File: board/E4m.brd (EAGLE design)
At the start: 49.4 x 100.1 mm, 76 parts, among them IC1 MCP23017SS, Q1 IRL540, Q2 IRL540, Q3 IRL540

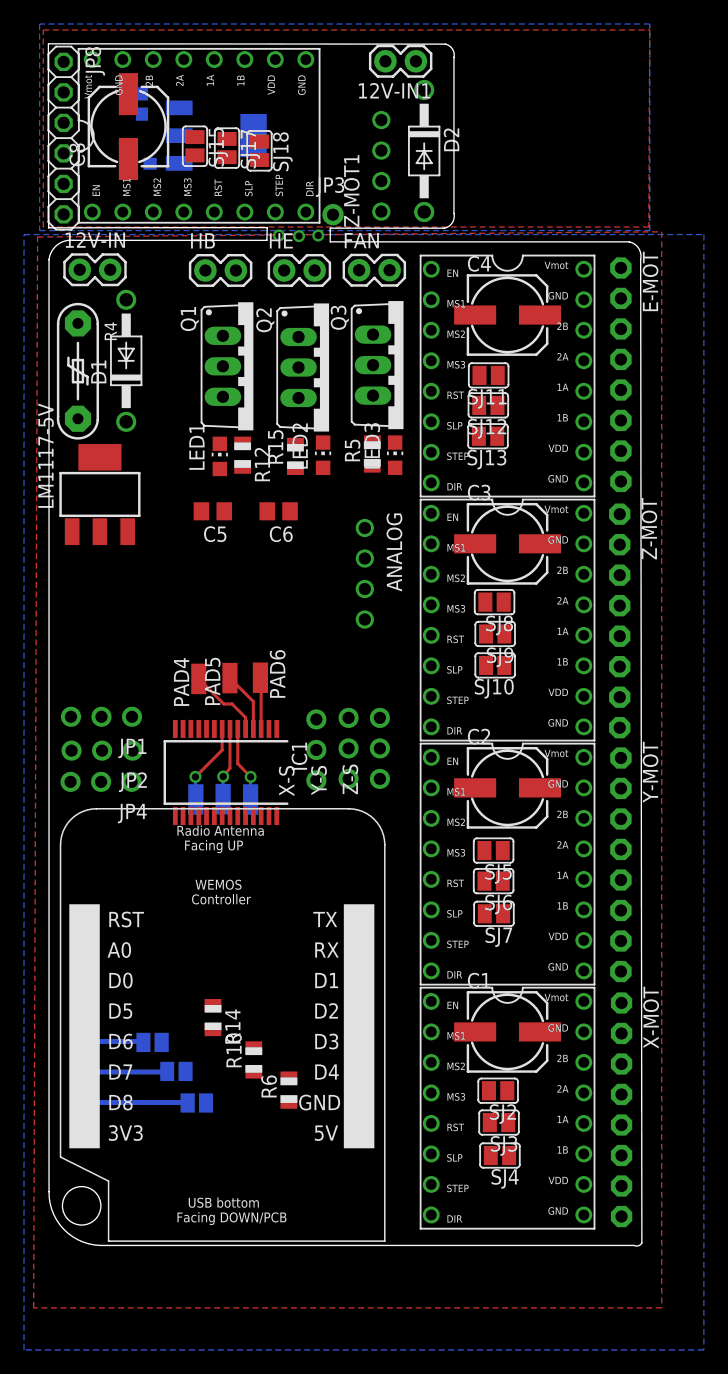
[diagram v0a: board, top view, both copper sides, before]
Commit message: 100% routed..... to clean before raster...
yup
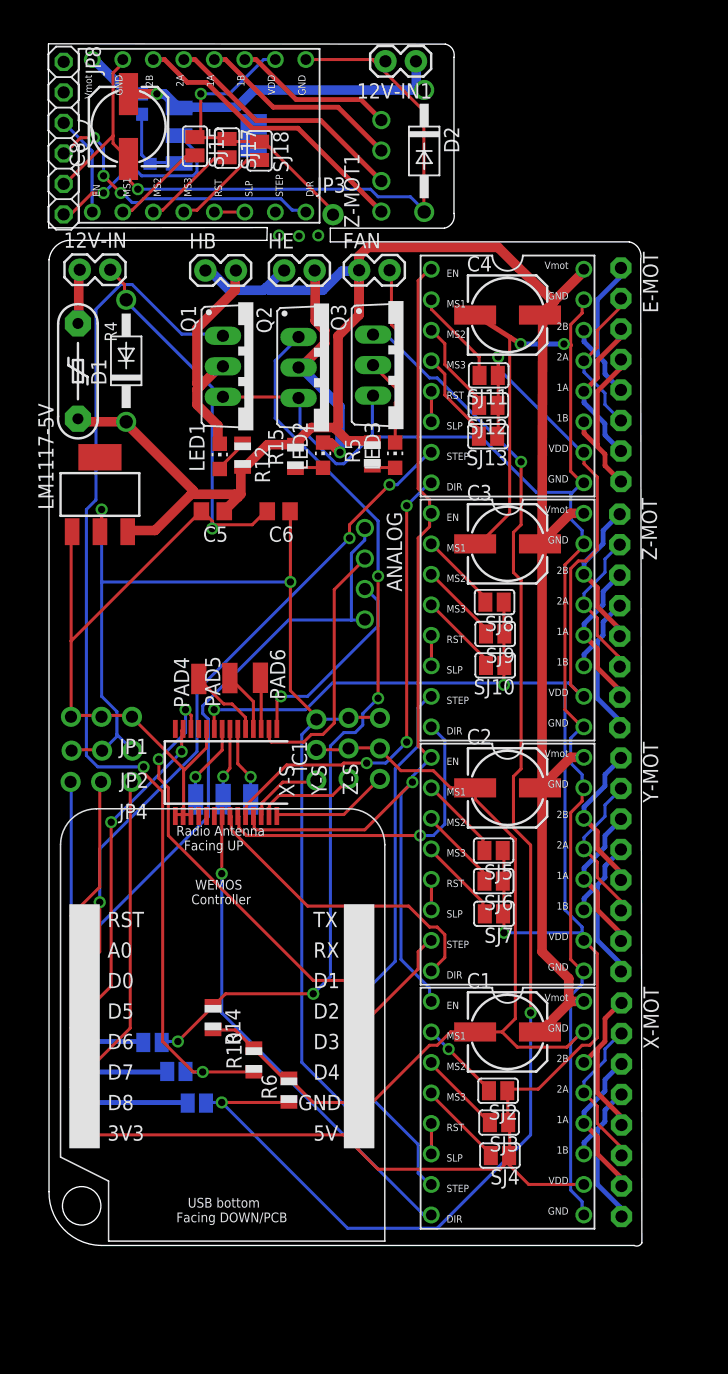
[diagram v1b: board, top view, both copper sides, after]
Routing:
- net GND: track 0.23 -> 310.8 mm, vias 0 -> 3
- net 3V3: track 0.18 -> 186.3 mm, vias 0 -> 4
- net 12V: track 0.00 -> 171.6 mm
- net N$27: track 0.00 -> 114.4 mm, vias 0 -> 3
- net 5V: track 0.00 -> 103.8 mm, vias 0 -> 2
- net N$S4: track 0.00 -> 89.5 mm, vias 0 -> 2
- net ENABLE: track 0.00 -> 81.1 mm, vias 0 -> 1
- net N$23: track 0.00 -> 76.2 mm, vias 0 -> 4
- net GND1: track 0.00 -> 63.6 mm, vias 0 -> 1
- net E-STEP: track 0.00 -> 56.5 mm, vias 0 -> 3
- net ANALOG: track 0.00 -> 49.5 mm
- net X-DIR: track 0.00 -> 40.8 mm, vias 0 -> 1
- net E-DIR: track 0.00 -> 39.0 mm, vias 0 -> 3
- net 12V1: track 0.00 -> 35.2 mm, vias 0 -> 1
- net SCL: track 0.00 -> 34.4 mm, vias 0 -> 2
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- removed copper zone on layer 1, net GND
- removed copper zone on layer 16, net GND
- removed copper zone on layer 1, net GND1
- removed copper zone on layer 16, net GND1
